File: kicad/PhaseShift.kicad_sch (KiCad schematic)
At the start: 40 parts

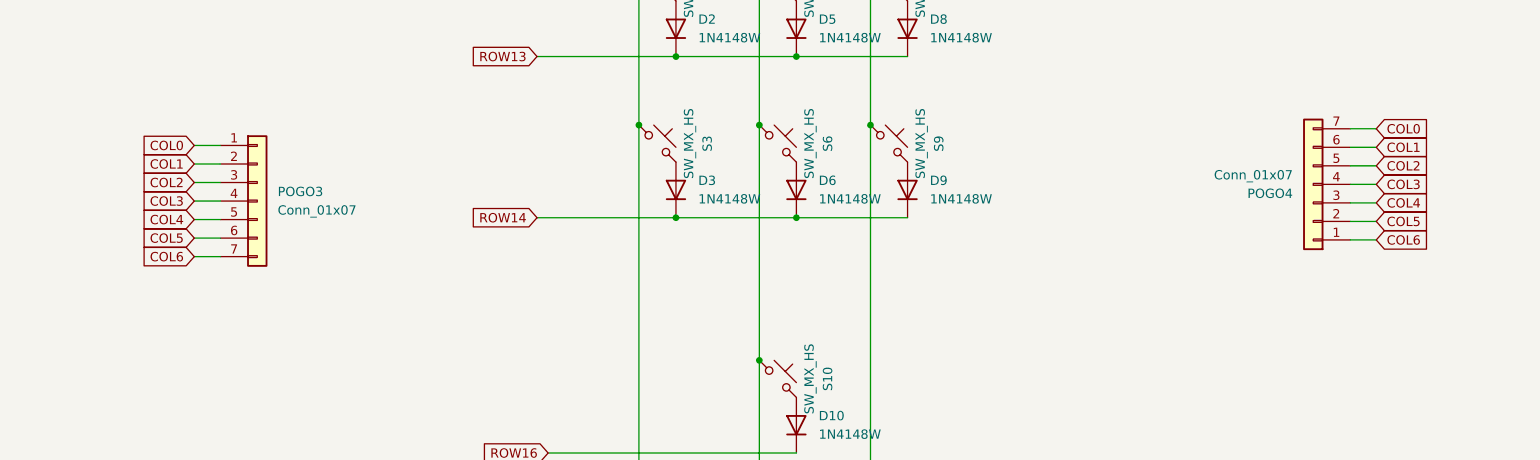
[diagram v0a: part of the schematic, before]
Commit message: quick fix
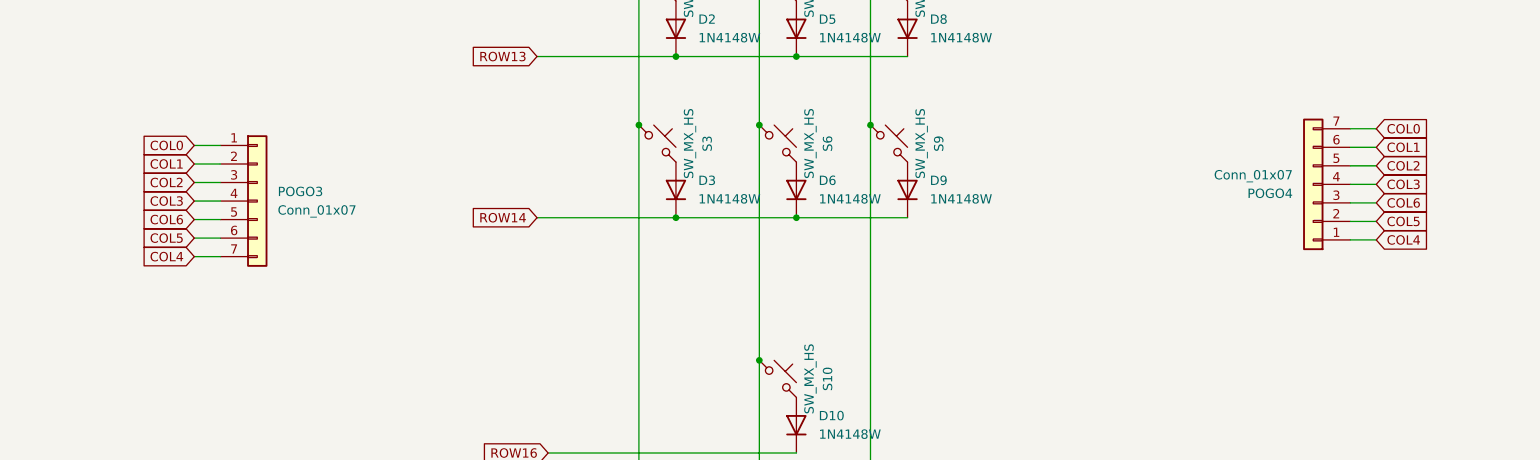
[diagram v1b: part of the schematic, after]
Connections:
- net COL4: now also POGO3.7 (Pin_7), POGO4.1 (Pin_1); no longer POGO3.5 (Pin_5), POGO4.3 (Pin_3)
- net COL6: now also POGO3.5 (Pin_5), POGO4.3 (Pin_3); no longer POGO3.7 (Pin_7), POGO4.1 (Pin_1)
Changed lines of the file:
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@@
+		)
+	)
+	(global_label "COL6"
+		(shape input)
+		(at 57.15 99.06 180)
+		(fields_autoplaced yes)
+		(effects
+			(font
+				(size 1.27 1.27)
+			)
+			(justify right)
+		)
+		(property "Intersheetrefs" "${INTERSHEET_REFS}"
+			(at 49.3267 99.06 0)
+			(effects
+				(font
+					(size 1.27 1.27)
+				)
+				(justify right)
+				(hide yes)
+			)
+		)
+	)
+	(global_label "COL3"
+		(shape input)
+		(at 57.15 96.52 180)
+		(fields_autoplaced yes)
+		(effects
+			(font
+				(size 1.27 1.27)
+			)
+			(justify right)
+		)
+		(property "Intersheetrefs" "${INTERSHEET_REFS}"
+			(at 49.3267 96.52 0)
+			(effects
+				(font
+					(size 1.27 1.27)
+				)
+				(justify right)
+				(hide yes)
+			)
+		)
+	)
+	(global_label "ROW16"
+		(shape input)
+		(at 218.948 145.034 0)
+		(fields_autoplaced yes)
+		(effects
+			(font
+				(size 1.27 1.27)
+			)
+			(justify left)
+		)
+		(property "Intersheetrefs" "${INTERSHEET_REFS}"
+			(at 228.4041 145.034 0)
+			(effects
+				(font
+					(size 1.27 1.27)
+				)
+				(justify left)
+				(hide yes)
+			)
+		)
+	)
+	(global_label "COL6"
+		(shape input)
+		(at 219.202 96.774 0)
+		(fields_autoplaced yes)
+		(effects
+			(font
+				(size 1.27 1.27)
+			)
+			(justify left)
+		)
+		(property "Intersheetrefs" "${INTERSHEET_REFS}"
+			(at 227.0253 96.774 0)
+			(effects
+				(font
+					(size 1.27 1.27)
+				)
+				(justify left)
+				(hide yes)
+			)
+		)
+	)
+	(global_label "+5V"
+		(shape input)
+		(at 57.15 59.182 180)
+		(fields_autoplaced yes)
+		(effects
+			(font
+				(size 1.27 1.27)
+			)
+			(justify right)
+		)
+		(property "Intersheetrefs" "${INTERSHEET_REFS}"
+			(at 50.2943 59.182 0)
+			(effects
+				(font
+					(size 1.27 1.27)
+				)
+				(justify right)
+				(hide yes)
+			)
+		)
+	)
+	(global_label "COL0"
+		(shape input)
+		(at 57.15 88.9 180)
+		(fields_autoplaced yes)
+		(effects
+			(font
+				(size 1.27 1.27)
+			)
+			(justify right)
+		)
+		(property "Intersheetrefs" "${INTERSHEET_REFS}"
+			(at 49.3267 88.9 0)
+			(effects
+				(font
+					(size 1.27 1.27)
+				)
+				(justify right)
+				(hide yes)
+			)
 		)
 	)
 	(global_label "COL4"
 		(shape input)
-		(at 57.15 99.06 180)
-		(fields_autoplaced yes)
-		(effects
-			(font
-				(size 1.27 1.27)
-			)
-			(justify right)
-		)
-		(property "Intersheetrefs" "${INTERSHEET_REFS}"
-			(at 49.3267 99.06 0)
-			(effects
-				(font
-					(size 1.27 1.27)
-				)
-				(justify right)
-				(hide yes)
-			)
-		)
-	)
-	(global_label "COL3"
-		(shape input)
-		(at 57.15 96.52 180)
-		(fields_autoplaced yes)
-		(effects
-			(font
-				(size 1.27 1.27)
-			)
-			(justify right)
-		)
-		(property "Intersheetrefs" "${INTERSHEET_REFS}"
-			(at 49.3267 96.52 0)
-			(effects
-				(font
-					(size 1.27 1.27)
-				)
-				(justify right)
-				(hide yes)
-			)
-		)
-	)
-	(global_label "ROW16"
-		(shape input)
-		(at 218.948 145.034 0)
-		(fields_autoplaced yes)
-		(effects
-			(font
-				(size 1.27 1.27)
-			)
-			(justify left)
-		)
-		(property "Intersheetrefs" "${INTERSHEET_REFS}"
-			(at 228.4041 145.034 0)
-			(effects
-				(font
-					(size 1.27 1.27)
-				)
-				(justify left)
+		(at 219.202 101.854 0)
+		(fields_autoplaced yes)
+		(effects
+			(font
+				(size 1.27 1.27)
+			)
+			(justify left)
+		)
+		(property "Intersheetrefs" "${INTERSHEET_REFS}"
+			(at 227.0253 101.854 0)
+			(effects
+				(font
+					(size 1.27 1.27)
+				)
+				(justify left)
+				(hide yes)
+			)
+		)
+	)
+	(global_label "RGB_FOM_LEFT"
+		(shape input)
+		(at 57.15 51.562 180)
+		(fields_autoplaced yes)
+		(effects
+			(font
+				(size 1.27 1.27)
+			)
+			(justify right)
+		)
+		(property "Intersheetrefs" "${INTERSHEET_REFS}"
+			(at 40.3158 51.562 0)
+			(effects
+				(font
+					(size 1.27 1.27)
+				)
+				(justify right)
+				(hide yes)
+			)
+		)
+	)
+	(global_label "RGB_FOM_RIGHT"
+		(shape input)
+		(at 218.948 150.114 0)
+		(fields_autoplaced yes)
+		(effects
+			(font
+				(size 1.27 1.27)
+			)
+			(justify left)
+		)
+		(property "Intersheetrefs" "${INTERSHEET_REFS}"
+			(at 236.9918 150.114 0)
+			(effects
+				(font
+					(size 1.27 1.27)
+				)
+				(justify left)
+				(hide yes)
+			)
+		)
+	)
+	(global_label "ROW13"
+		(shape input)
+		(at 104.14 76.708 180)
+		(fields_autoplaced yes)
+		(effects
+			(font
+				(size 1.27 1.27)
+			)
+			(justify right)
+		)
+		(property "Intersheetrefs" "${INTERSHEET_REFS}"
+			(at 94.6839 76.708 0)
+			(effects
+				(font
+					(size 1.27 1.27)
+				)
+				(justify right)
 				(hide yes)
 			)
@@
 	(global_label "COL4"
 		(shape input)
-		(at 219.202 96.774 0)
-		(fields_autoplaced yes)
-		(effects
-			(font
-				(size 1.27 1.27)
-			)
-			(justify left)
-		)
-		(property "Intersheetrefs" "${INTERSHEET_REFS}"
-			(at 227.0253 96.774 0)
-			(effects
-				(font
-					(size 1.27 1.27)
-				)
-				(justify left)
-				(hide yes)
-			)
-		)
-	)
-	(global_label "+5V"
-		(shape input)
-		(at 57.15 59.182 180)
-		(fields_autoplaced yes)
-		(effects
-			(font
-				(size 1.27 1.27)
-			)
-			(justify right)
-		)
-		(property "Intersheetrefs" "${INTERSHEET_REFS}"
-			(at 50.2943 59.182 0)
-			(effects
-				(font
-					(size 1.27 1.27)
-				)
-				(justify right)
-				(hide yes)
-			)
-		)
-	)
-	(global_label "COL0"
-		(shape input)
-		(at 57.15 88.9 180)
-		(fields_autoplaced yes)
-		(effects
-			(font
-				(size 1.27 1.27)
-			)
-			(justify right)
-		)
-		(property "Intersheetrefs" "${INTERSHEET_REFS}"
-			(at 49.3267 88.9 0)
-			(effects
-				(font
-					(size 1.27 1.27)
-				)
-				(justify right)
-				(hide yes)
-			)
-		)
-	)
-	(global_label "COL6"
-		(shape input)
-		(at 219.202 101.854 0)
-		(fields_autoplaced yes)
-		(effects
-			(font
-				(size 1.27 1.27)
-			)
-			(justify left)
-		)
-		(property "Intersheetrefs" "${INTERSHEET_REFS}"
-			(at 227.0253 101.854 0)
-			(effects
-				(font
-					(size 1.27 1.27)
-				)
-				(justify left)
-				(hide yes)
-			)
-		)
-	)
-	(global_label "RGB_FOM_LEFT"
-		(shape input)
-		(at 57.15 51.562 180)
-		(fields_autoplaced yes)
-		(effects
-			(font
-				(size 1.27 1.27)
-			)
-			(justify right)
-		)
-		(property "Intersheetrefs" "${INTERSHEET_REFS}"
-			(at 40.3158 51.562 0)
-			(effects
-				(font
-					(size 1.27 1.27)
-				)
-				(justify right)
-				(hide yes)
-			)
-		)
-	)
-	(global_label "RGB_FOM_RIGHT"
-		(shape input)
-		(at 218.948 150.114 0)
-		(fields_autoplaced yes)
-		(effects
-			(font
-				(size 1.27 1.27)
-			)
-			(justify left)
-		)
-		(property "Intersheetrefs" "${INTERSHEET_REFS}"
-			(at 236.9918 150.114 0)
-			(effects
-				(font
-					(size 1.27 1.27)
-				)
-				(justify left)
-				(hide yes)
-			)
-		)
-	)
-	(global_label "ROW13"
-		(shape input)
-		(at 104.14 76.708 180)
-		(fields_autoplaced yes)
-		(effects
-			(font
-				(size 1.27 1.27)
-			)
-			(justify right)
-		)
-		(property "Intersheetrefs" "${INTERSHEET_REFS}"
-			(at 94.6839 76.708 0)
-			(effects
-				(font
-					(size 1.27 1.27)
-				)
-				(justify right)
-				(hide yes)
-			)
-		)
-	)
-	(global_label "COL6"
-		(shape input)
 		(at 57.15 104.14 180)
